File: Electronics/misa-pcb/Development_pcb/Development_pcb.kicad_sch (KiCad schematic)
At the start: 30 parts, among them J1 Pan-Servo, J2 Tilt-Servo, J3 cam-power, J4 laser-power, J5 SPEAKER, J6 TFT_display, J7 lidar-TOF, J8 USB_C_IN, Q1 PN2222A, U1 ESP32-S3-DEVKITC-1-N8R8, U2 MP3-TF-16P

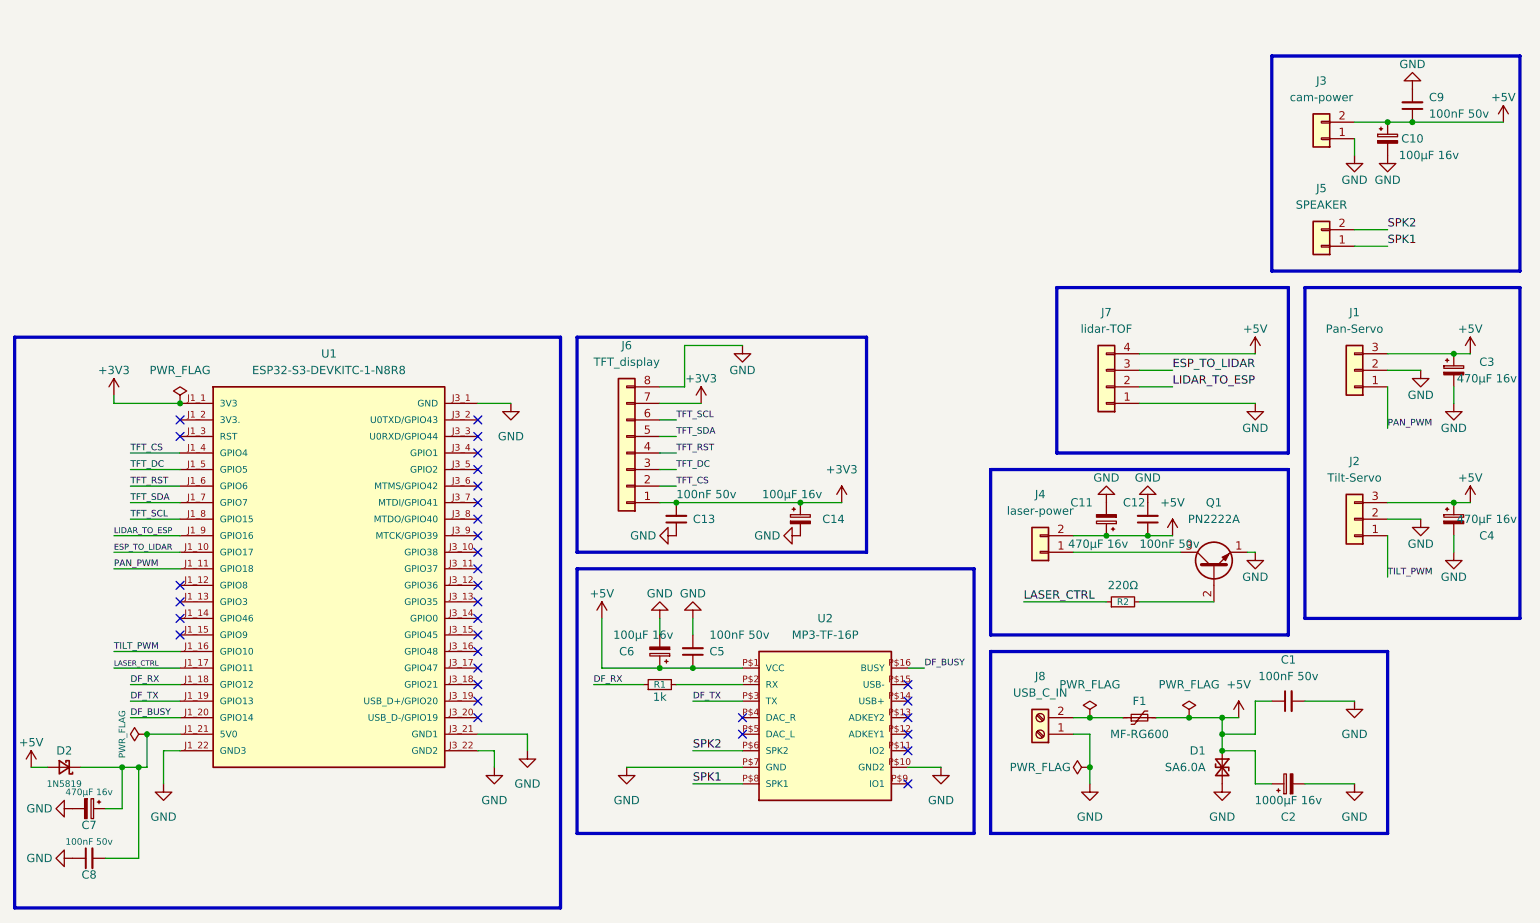
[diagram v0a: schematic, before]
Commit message: Refactor code structure and remove redundant sections for improved readability and maintainability
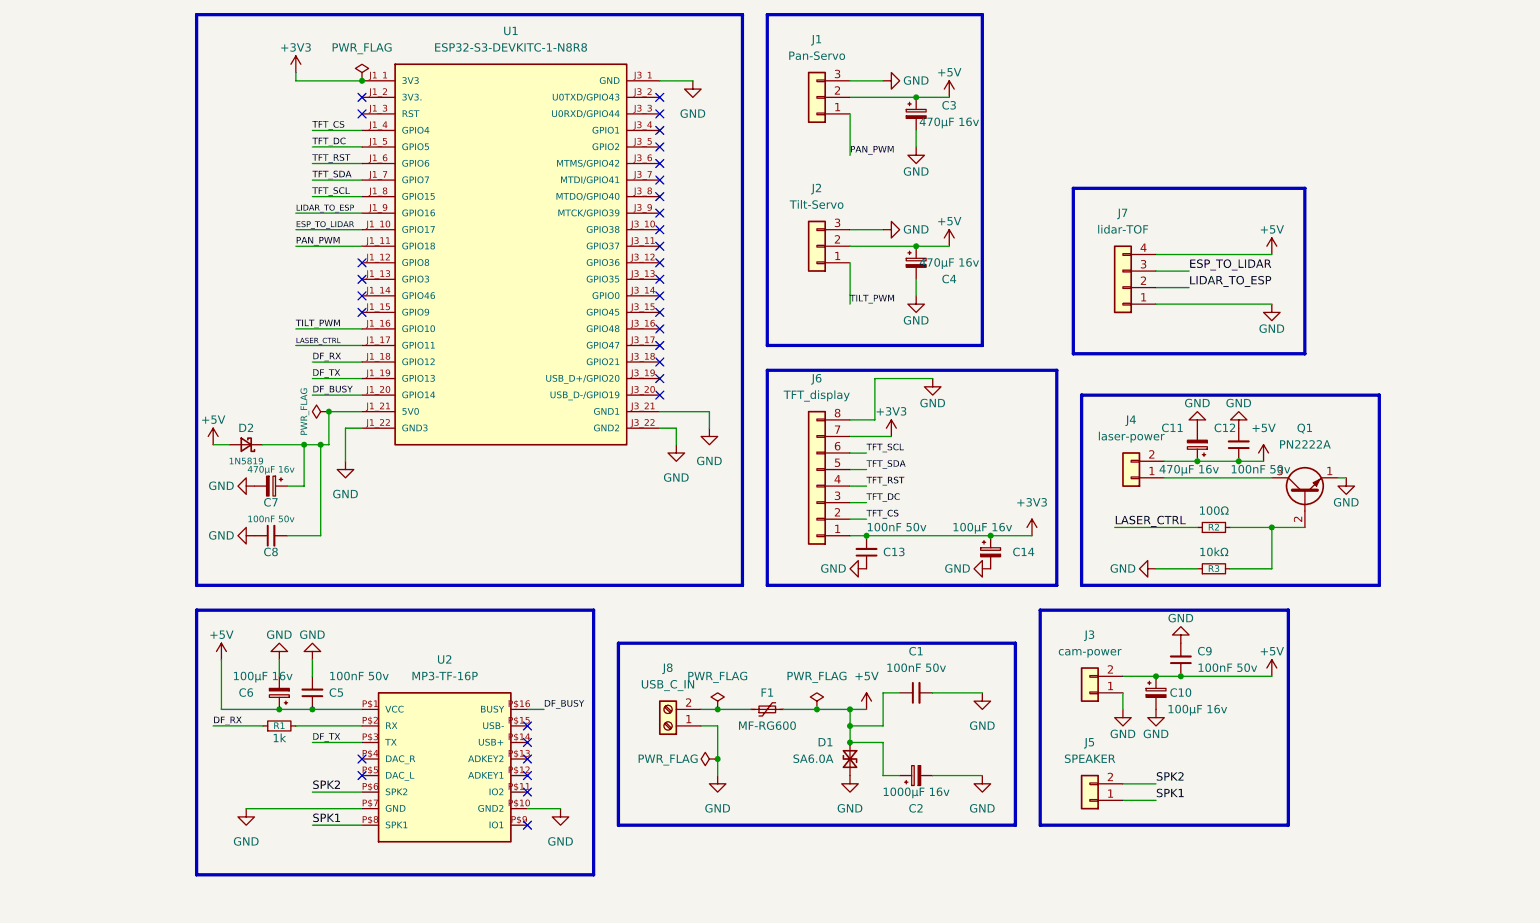
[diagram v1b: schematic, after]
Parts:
- added R3: 10kΩ, Resistor_THT:R_Axial_DIN0207_L6.3mm_D2.5mm_P2.54mm_Vertical, symbol Device:R_Small
- C10, C6: footprint Capacitor_THT:CP_Radial_D5.0mm_P2.50mm -> Capacitor_THT:CP_Radial_D6.3mm_P2.50mm
- R2: value 220Ω -> 100Ω
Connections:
- net +5V: now also J1.2 (Pin_2), J2.2 (Pin_2); no longer J1.3 (Pin_3), J2.3 (Pin_3)
- net GND: now also J1.3 (Pin_3), J2.3 (Pin_3), R3.1; no longer J1.2 (Pin_2), J2.2 (Pin_2)
- net at Q1.2 (B), R2.2: now also R3.2
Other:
- moved on the sheet: C1, C10, C11, C12, C13, C14, C2, C3, C4, C5, C6, C7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
